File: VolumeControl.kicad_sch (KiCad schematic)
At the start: 15 parts

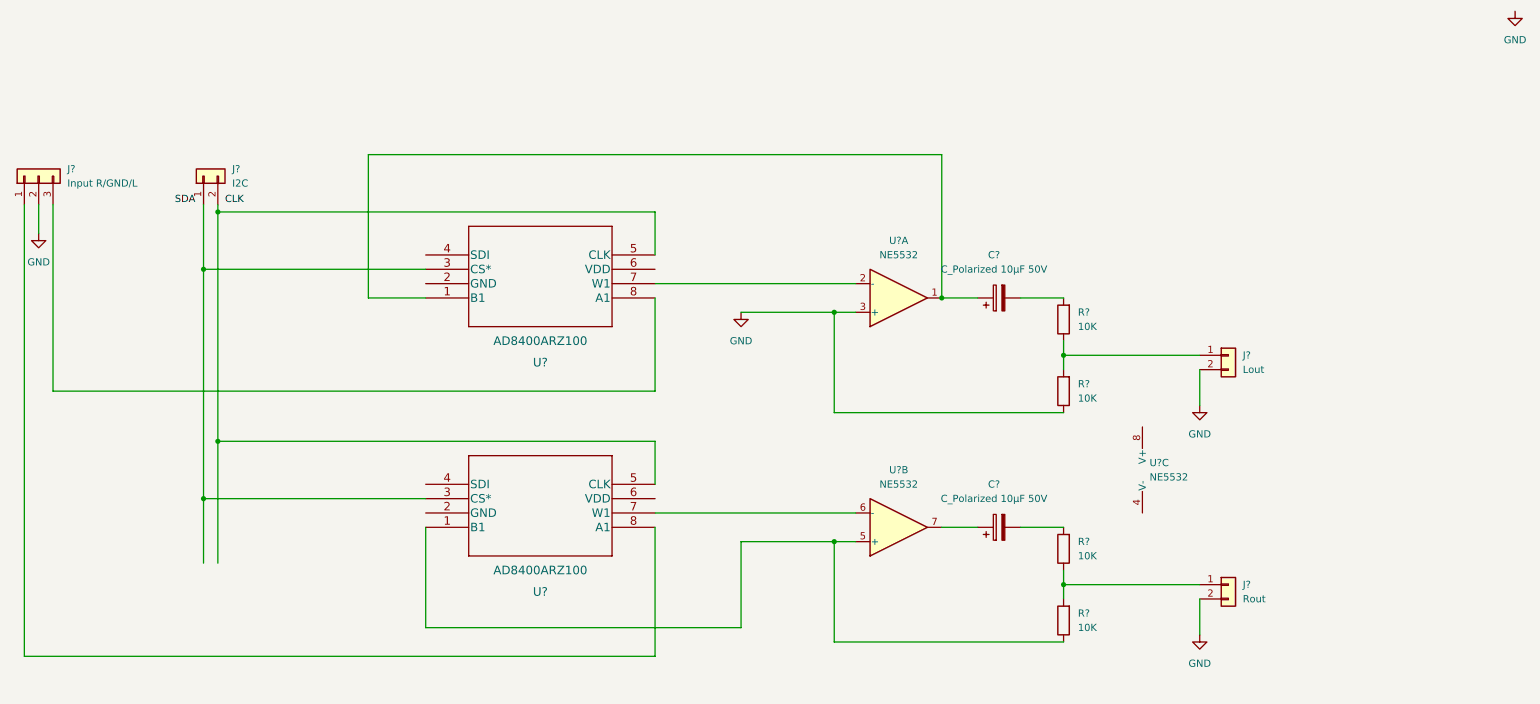
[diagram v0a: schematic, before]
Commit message: some corrections
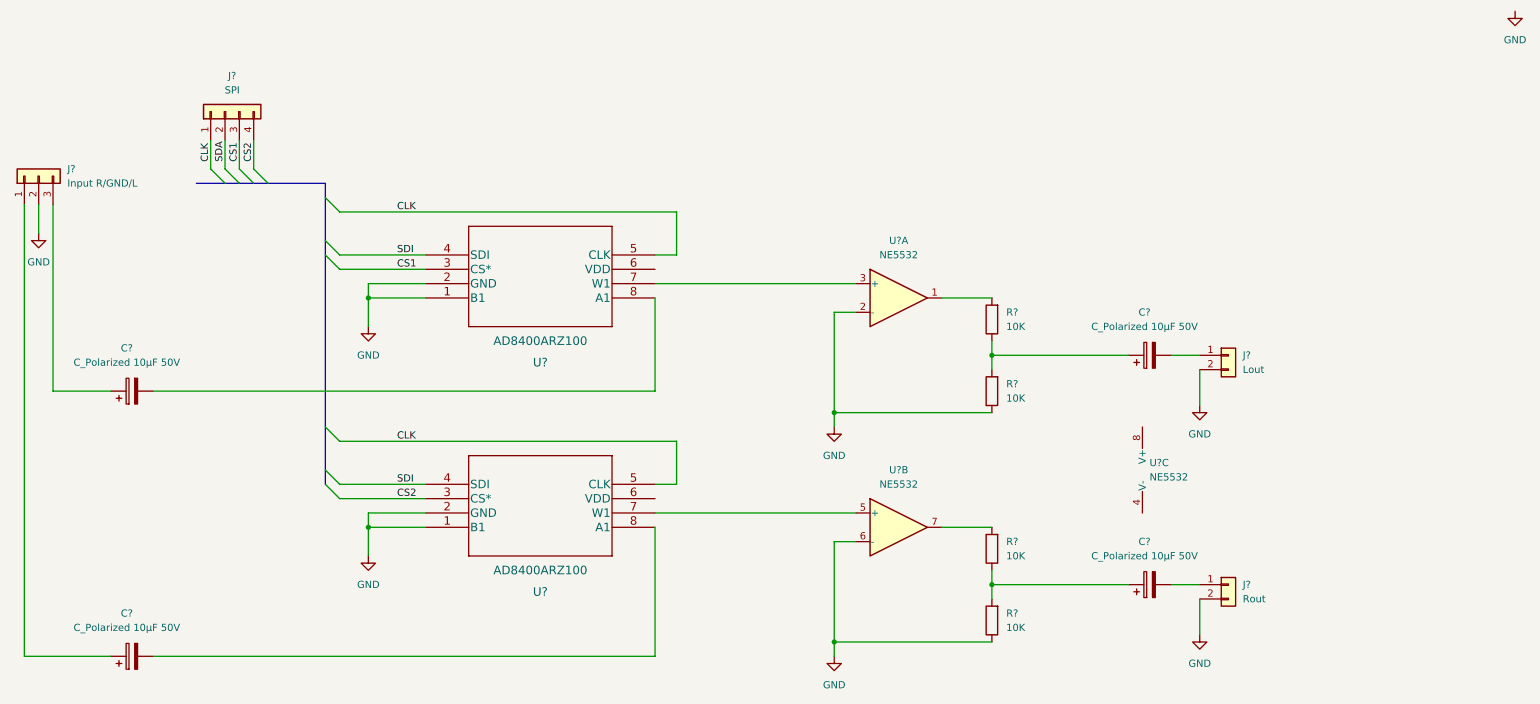
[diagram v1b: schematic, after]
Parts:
- added C? (x2): C_Polarized 10µF 50V, symbol Device:C_Polarized
- J?: value I2C -> SPI; symbol Connector_Generic:Conn_01x02 -> Connector_Generic:Conn_01x04
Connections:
- net CLK: now also J?.1 (Pin_1), U?.5 (CLK), U?.5 (CLK)
- net GND: now also R?.1, U?.1 (B1), U?.1 (B1), U?.2 (-), U?.2 (GND), U?.2 (GND), U?.6 (-); no longer U?.3 (+)
- net SDA: now also J?.2 (Pin_2)
- net at R?.1, R?.2: now also C?.1; no longer J?.1 (Pin_1) (x2)
- net at J?.1 (Pin_1): now also C?.1; no longer U?.8 (A1)
- net at J?.3 (Pin_3): now also C?.1; no longer U?.8 (A1)
- net at C?.2: now also J?.1 (Pin_1); no longer R?.2 (x2)
- net at U?.7 (W1): now also U?.3 (+); no longer U?.2 (-)
- net SDI: now reaches U?.4 (SDI)
- net SDI: now also U?.4 (SDI)
- net at U?.7 (W1): now also U?.5 (+); no longer U?.6 (-)
- net at U?.7: now also R?.2; no longer C?.1
- new net: C?.2, U?.8 (A1) (x2)
- new net: R?.2, U?.1
- new net CS1: J?.3 (Pin_3), U?.3 (CS*)
- new net CS2: J?.4 (Pin_4), U?.3 (CS*)
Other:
- moved on the sheet: C?, R?
